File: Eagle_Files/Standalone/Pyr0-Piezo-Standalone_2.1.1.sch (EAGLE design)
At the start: 71 parts, among them J1 FFC-15P-1MM, U1 ATMEGA48/88/168/328PA, U4 LM2902QT, X1 FFC-40P-0.5SH

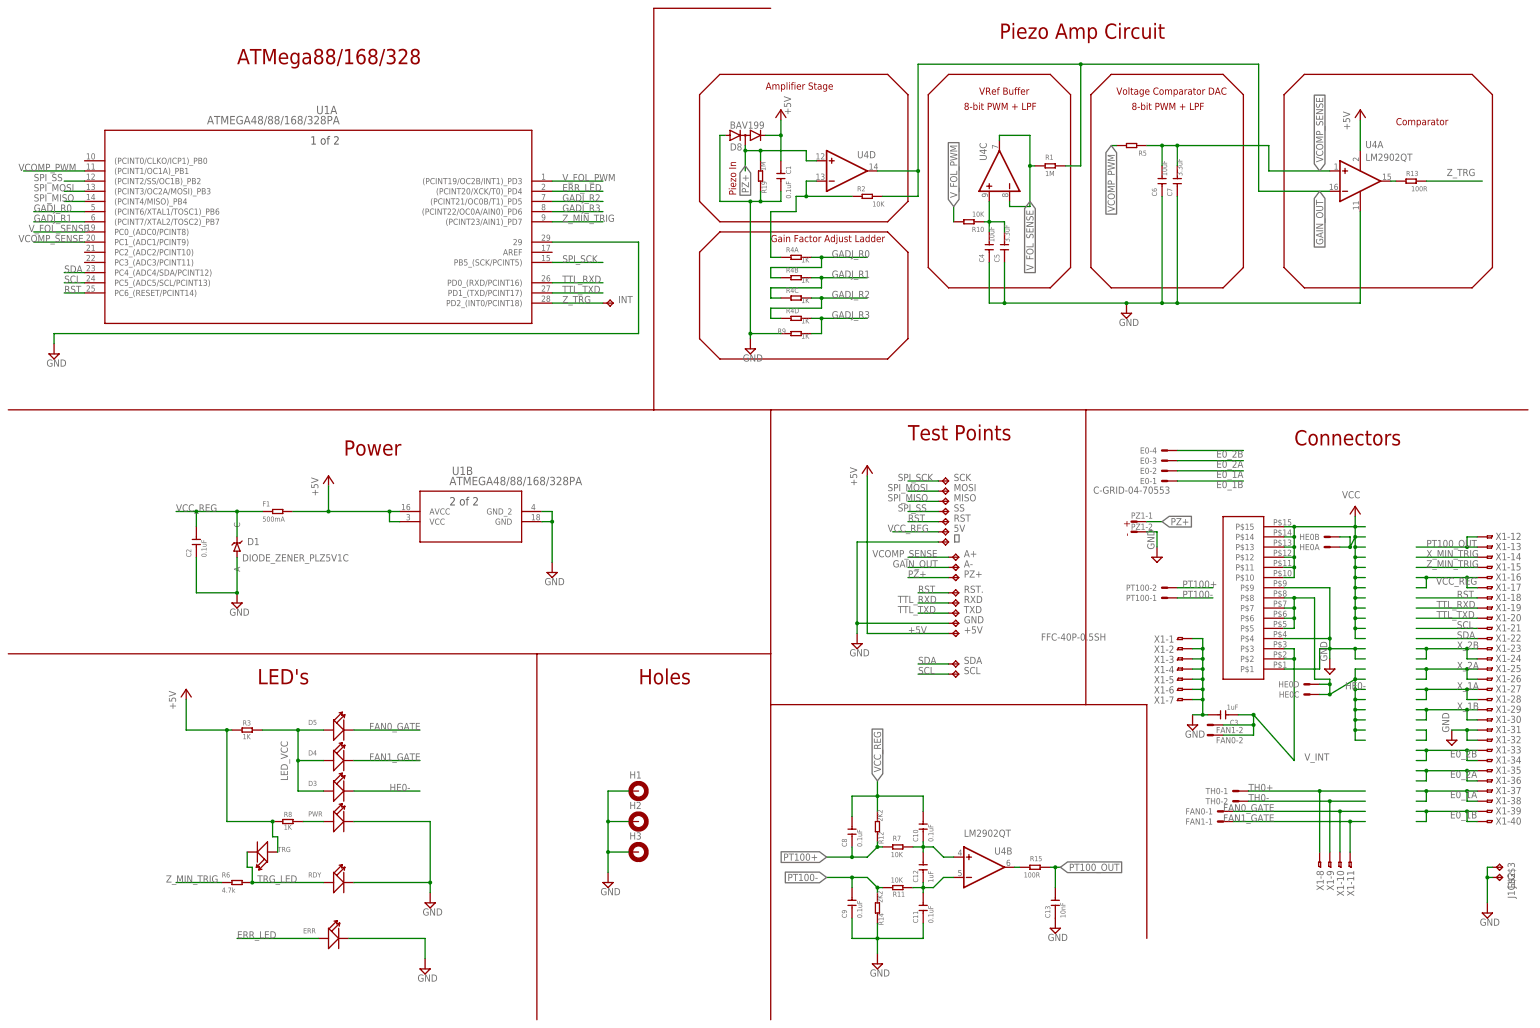
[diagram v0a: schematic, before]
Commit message: fixed some file encoding issues
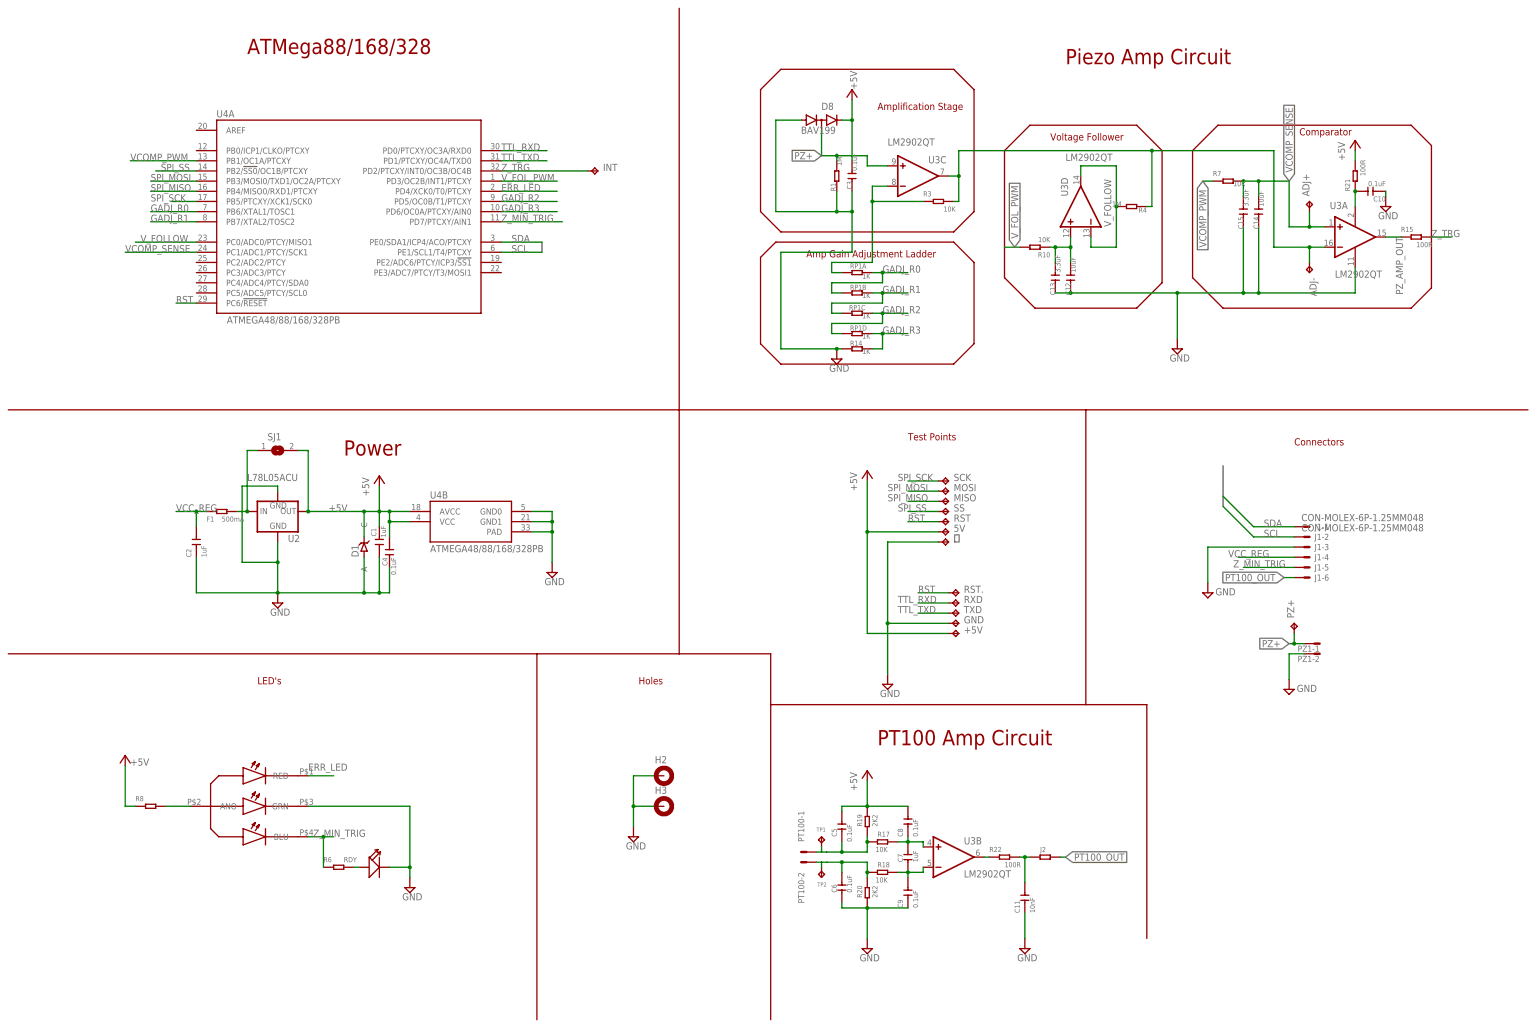
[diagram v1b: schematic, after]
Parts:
- removed A+, A-: TPTP13SQ, PiezoFFC:TPTP13SQ
- removed D3, D4, D5, ERR, PWR, TRG: (no value), PiezoFFC:SEEED-LED_SMD-LED-CLEAR-BLUE(0603)LED_0603
- removed E0: C-GRID-04-70553, PiezoFFC:C-GRID-04-70553
- removed FAN0, FAN1, TH0: CON-MOLEX-2P-1.27MM048, PiezoFFC:CON-MOLEX-2P-1.27MM048
- removed H1: HOLES_MOUNT-PAD-ROUND3.2, PiezoFFC:HOLES_MOUNT-PAD-ROUND3.2
- removed HE0: JST-2.54-2X2JST-DUPONT-2.54-2X2, PiezoFFC:JST-2.54-2X2JST-DUPONT-2.54-2X2
- removed R11, R2: 10K, PiezoFFC:SMD-RES-0R-5%-1/16W(0402)
- removed R12: 2K2, PiezoFFC:SMD-RES-0R-5%-1/16W(0402)
- removed R13: 100R, PiezoFFC:SMD-RES-0R-5%-1/16W(0402)
- removed R5: 10K, PiezoFFC:SEEED-RESISTOR_SMD-RES-1.5K-1%-1/10W(0603)DETAILED_MODEL
- removed R9: 1K, PiezoFFC:SMD-RES-0R-5%-1/16W(0402)
- removed SCL, SDA: TPTP13SQ, testpad:TPTP13SQ
- removed U1: ATMEGA48/88/168/328PA, PiezoFFC:ATMEGA48/88/168/328PA
- removed X1: FFC-40P-0.5SH, PiezoFFC:FFC-40P-0.5SH
- added ADJ+, ADJ-: TPTP13SQ, PiezoFFC:TPTP13SQ
- added C14: 10uF, PiezoFFC:CERAMIC-1NF-50V-10%-X7R(0402)CAP_0402
- added C15: 3.3uF, PiezoFFC:CERAMIC-1NF-50V-10%-X7R(0402)CAP_0402
- added J2: (no value), PiezoFFC:SEEED-RESISTOR_SMD-RES-1.5K-1%-1/10W(0603)DETAILED_MODEL
- added LED: LED-RGB-COM_ANO0606, PiezoFFC:LED-RGB-COM_ANO0606
- added R17, R18: 10K, PiezoFFC:SMD-RES-0R-5%-1/16W(0402)
- added R20: 2K2, PiezoFFC:SMD-RES-0R-5%-1/16W(0402)
- added R21, R22: 100R, PiezoFFC:SMD-RES-0R-5%-1/16W(0402)
- added RP1: 1K, PiezoFFC:RESISTOR_NETWORK_X40804_L
- added SJ1: (no value), PiezoFFC:SJM
- added TP1, TP2: TPTP09R, PiezoFFC:TPTP09R
- added U2: L78L05ACU, PiezoFFC:L78L05ACU
- added U3: LM2902QT, PiezoFFC:LM2902QT
- C1, C2: value 0.1uF -> 1uF; device PiezoFFC:CERAMIC-1NF-50V-10%-X7R(0402)CAP_0402 -> PiezoFFC:SEEED-CAPACITOR_CERAMIC-10UF-25V-10%-X5R(0805)CAP_0603_GEN
- C11: value 0.1uF -> 10nF
- C12: value 1uF -> 10uF
- C13: value 10nF -> 3.3uF
- C3: value 1uF -> 0.1uF; device PiezoFFC:SEEED-CAPACITOR_CERAMIC-10UF-25V-10%-X5R(0805)CAP_0603_GEN -> PiezoFFC:CERAMIC-1NF-50V-10%-X7R(0402)CAP_0402
- C4, C6: value 10uF -> 0.1uF
- C5: value 3.3uF -> 0.1uF; device PiezoFFC:SEEED-CAPACITOR_CERAMIC-10UF-25V-10%-X5R(0805)CAP_0603_GEN -> PiezoFFC:CERAMIC-1NF-50V-10%-X7R(0402)CAP_0402
- C7: value 3.3uF -> 1uF; device PiezoFFC:SEEED-CAPACITOR_CERAMIC-10UF-25V-10%-X5R(0805)CAP_0603_GEN -> PiezoFFC:CERAMIC-1NF-50V-10%-X7R(0402)CAP_0402
- F1: device PiezoFFC:SEEED-RESISTOR_SMD-RES-1.5K-1%-1/10W(0603)DETAILED_MODEL -> PiezoFFC:SMD-RES-0R-5%-1/16W(0402)
- H2, H3: value HOLES_MOUNT-PAD-ROUND3.2 -> HOLES_MOUNT-PAD-ROUND2.8; device PiezoFFC:HOLES_MOUNT-PAD-ROUND3.2 -> PiezoFFC:HOLES_MOUNT-PAD-ROUND2.8
- J1: value FFC-15P-1MM -> CON-MOLEX-6P-1.25MM048; device PiezoFFC:FFC-15P-1MM -> PiezoFFC:CON-MOLEX-6P-1.25MM048
- R14: value 2K2 -> 1K
- R19: value 1M -> 2K2
- R3: value 1K -> 10K
- R4: value 1K -> 1M; device PiezoFFC:RESISTOR_NETWORK_X40804 -> PiezoFFC:SMD-RES-0R-5%-1/16W(0402)
- R6: value 4.7k -> (none)
- R8: value 1K -> (none)
- U4: value LM2902QT -> ATMEGA48/88/168/328PB; device PiezoFFC:LM2902QT -> PiezoFFC:ATMEGA48/88/168/328PB
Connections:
- removed net E0_1A: E0-2.S, X1-37.1, X1-38.1
- removed net E0_1B: E0-1.S, X1-39.1, X1-40.1
- removed net E0_2A: E0-3.S, X1-35.1, X1-36.1
- removed net E0_2B: E0-4.S, X1-33.1, X1-34.1
- removed net FAN0_GATE: D5.-, FAN0-1.S, X1-10.1
- removed net FAN1_GATE: D4.-, FAN1-1.S, X1-11.1
- removed net GAIN_FB: R2.1, R4A.1, U4D.-IN
- removed net HE0-: D3.-, HE0C.S, HE0D.S, J1G$1.P$5, J1G$1.P$6, J1G$1.P$7, J1G$1.P$8
- removed net LED_VCC: D3.+, D4.+, D5.+, R3.2
- removed net N$2: PWR.+, R8.2
- removed net PT100+: C8.1, PT100-2.S, R12.1, R7.2
- removed net PT100-: C9.2, PT100-1.S, R11.2, R14.2
- removed net PT100_AMP+: C10.1, C12.2, R7.1, U4B.+IN
- removed net PT100_AMP-: C11.2, C12.1, R11.1, U4B.-IN
- removed net PT100_R: R15.2, U4B.OUT
- removed net TH0+: TH0-1.S, X1-8.1
- removed net TH0-: TH0-2.S, X1-9.1
- removed net TRG_LED: R6.2, RDY.+, TRG.-
- removed net VCC: HE0A.S, HE0B.S, J1G$1.P$10, J1G$1.P$11, J1G$1.P$12, J1G$1.P$13, J1G$1.P$14, J1G$1.P$15
- removed net VREF_IN: C4.2, C5.2, R10.1, U4C.+IN
- removed net V_FOL_SENSE: R1.1, U1A.PC0_(ADC0/PCINT8), U4C.-IN, U4C.OUT
- removed net V_INT: C3.1, FAN0-2.S, FAN1-2.S, J1G$1.P$2, J1G$1.P$3
- removed net X_1A: X1-27.1, X1-28.1
- removed net X_1B: X1-29.1, X1-30.1
- removed net X_2A: X1-25.1, X1-26.1
- removed net X_2B: X1-23.1, X1-24.1
- removed net X_MIN_TRIG: X1-14.1
- new net AMP_VCC: C10.2, R21.1, U3P.V+
- new net GAIN_ADJ: R3.1, RP1A.1, U3C.-IN
- new net LED_PWR: LED.ANO, R8.2
- new net PT100_JUMP: C11.2, J2.1, R22.2
- new net PT_AMP: R22.1, U3B.OUT
- new net PT_AMP+: C7.2, C8.1, R17.2, U3B.+IN
- new net PT_AMP-: C7.1, C9.2, R18.2, U3B.-IN
- new net PT_IN+: C5.1, PT100-1.S, R17.1, R19.1, TP1.TP
- new net PT_IN-: C6.2, PT100-2.S, R18.1, R20.2, TP2.TP
- new net RDY_LED: R6.2, RDY.+
- new net VCC_FUSE: F1.2, SJ1.1, U2.IN
- new net V_FOLLOW: R4.2, U3D.-IN, U3D.OUT, U4A.PC0/ADC0/PTCY/MISO1
- new net V_FOL_ADJ: C12.2, C13.2, R10.1, U3D.+IN
- net +5V: now also 5V.TP, C1.2, C3.2, C4.2, C5.2, C8.2, D1.C, R19.2, R21.2, SJ1.2, U2.OUT, U4B.AVCC, U4B.VCC; no longer C1.1, F1.2, R3.1, TRG.+, U1B.AVCC, U1B.VCC, U4P.V+
- net ERR_LED: now also LED.RED, U4A.PD4/XCK0/T0/PTCXY; no longer ERR.+, U1A.(PCINT20/XCK/T0)_PD4
- net GADJ_R0: now also RP1A.2, RP1B.1, U4A.PB6/XTAL1/TOSC1; no longer R4A.2, R4B.1, U1A.(PCINT6/XTAL1/TOSC1)_PB6
- net GADJ_R1: now also RP1B.2, RP1C.1, U4A.PB7/XTAL2/TOSC2; no longer R4B.2, R4C.1, U1A.(PCINT7/XTAL2/TOSC2)_PB7
- net GADJ_R2: now also RP1C.2, RP1D.1, U4A.PD5/OC0B/T1/PTCXY; no longer R4C.2, R4D.1, U1A.(PCINT21/OC0B/T1)_PD5
- net GADJ_R3: now also R14.2, RP1D.2, U4A.PD6/OC0A/PTCXY/AIN0; no longer R4D.2, R9.2, U1A.(PCINT22/OC0A/AIN0)_PD6
- net GAIN_OUT: now also ADJ-.TP, R3.2, R4.1, U3A.-IN, U3C.OUT; no longer A-.TP, R1.2, R2.2, U4A.-IN, U4D.OUT
- net GND: now also C1.1, C10.1, C12.1, C14.1, C15.1, C3.1, J1-3.S, LED.GRN, R1.1, R20.1, U2.GND, U2.PAD, U3P.V-, U4B.GND0, U4B.GND1, U4B.PAD; no longer C1.2, C3.2, C5.1, C7.1, ERR.-, H1.MOUNT, J1G$1.P$1, J1G$1.P$4, J1G$1.P$9, J1G$2.TP, J1G$3.TP, PWR.-, R19.1, R9.1, U1A.29, U1B.GND, U1B.GND_2, U4P.V-, X1-1.1, X1-2.1, X1-3.1, X1-31.1, X1-32.1, X1-4.1, X1-5.1, X1-6.1, X1-7.1
- net PT100_OUT: now also J1-6.S, J2.2; no longer C13.2, R15.1, X1-12.1, X1-13.1
- net PZ+: now also R1.2, U3C.+IN; no longer R19.2, U4D.+IN
- net PZ_AMP_OUT: now also R15.1, U3A.OUT; no longer R13.1, U4A.OUT
- net RST: now also U4A.PC6/!RESET!; no longer U1A.PC6_(RESET/PCINT14), X1-18.1
- net SCL: now also J1-2.S, U4A.PE1/SCL1/T4/PTCXY; no longer SCL.TP, U1A.PC5_(ADC5/SCL/PCINT13), X1-21.1
- net SDA: now also J1-1.S, U4A.PE0/SDA1/ICP4/ACO/PTCXY; no longer SDA.TP, U1A.PC4_(ADC4/SDA/PCINT12), X1-22.1
- net SPI_MISO: now also U4A.PB4/MISO0/RXD1/PTCXY; no longer U1A.(PCINT4/MISO)_PB4
- net SPI_MOSI: now also U4A.PB3/MOSI0/TXD1/OC2A/PTCXY; no longer U1A.(PCINT3/OC2A/MOSI)_PB3
- net SPI_SCK: now also U4A.PB5/PTCXY/XCK1/SCK0; no longer U1A.PB5_(SCK/PCINT5)
- net SPI_SS: now also U4A.PB2/!SS0!/OC1B/PTCXY; no longer U1A.(PCINT2/SS/OC1B)_PB2
- net TTL_RXD: now also U4A.PD0/PTCXY/OC3A/RXD0; no longer U1A.PD0_(RXD/PCINT16), X1-19.1
- net TTL_TXD: now also U4A.PD1/PTCXY/OC4A/TXD0; no longer U1A.PD1_(TXD/PCINT17), X1-20.1
- net VCC_REG: now also J1-4.S; no longer 5V.TP, C10.2, C8.2, D1.C, R12.2, X1-16.1, X1-17.1
- net VCOMP_PWM: now also R7.1, U4A.PB1/OC1A/PTCXY; no longer R5.2, U1A.(PCINT1/OC1A)_PB1
- net VCOMP_SENSE: now also ADJ+.TP, C14.2, C15.2, R7.2, U3A.+IN, U4A.PC1/ADC1/PTCY/SCK1; no longer A+.TP, C6.2, C7.2, R5.1, U1A.PC1_(ADC1/PCINT9), U4A.+IN
- net V_FOL_PWM: now also U4A.PD3/OC2B/INT1/PTCXY; no longer U1A.(PCINT19/OC2B/INT1)_PD3
- net Z_MIN_TRIG: now also J1-5.S, LED.BLU, U4A.PD7/PTCXY/AIN1; no longer U1A.(PCINT23/AIN1)_PD7, X1-15.1
- net Z_TRG: now also R15.2, U4A.PD2/PTCXY/INT0/OC3B/OC4B; no longer R13.2, U1A.PD2_(INT0/PCINT18)
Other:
- note added: "Amp Gain Adjustment Ladder"
- note added: "Amplification Stage"
- note added: "PT100 Amp Circuit"
- note added: "Voltage Follower"
- note removed: "- +"
- note removed: "8-bit PWM + LPF"
- note removed: "Amplifier Stage"
- note removed: "Gain Factor Adjust Ladder"
- note removed: "Piezo In"
- note removed: "VRef Buffer"
- note removed: "Voltage Comparator DAC"
- moved on the sheet: C1, C10, C11, C12, C13, C3, C4, C5, C6, C7, C8, C9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
